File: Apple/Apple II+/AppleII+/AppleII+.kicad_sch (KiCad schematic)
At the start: 0 parts

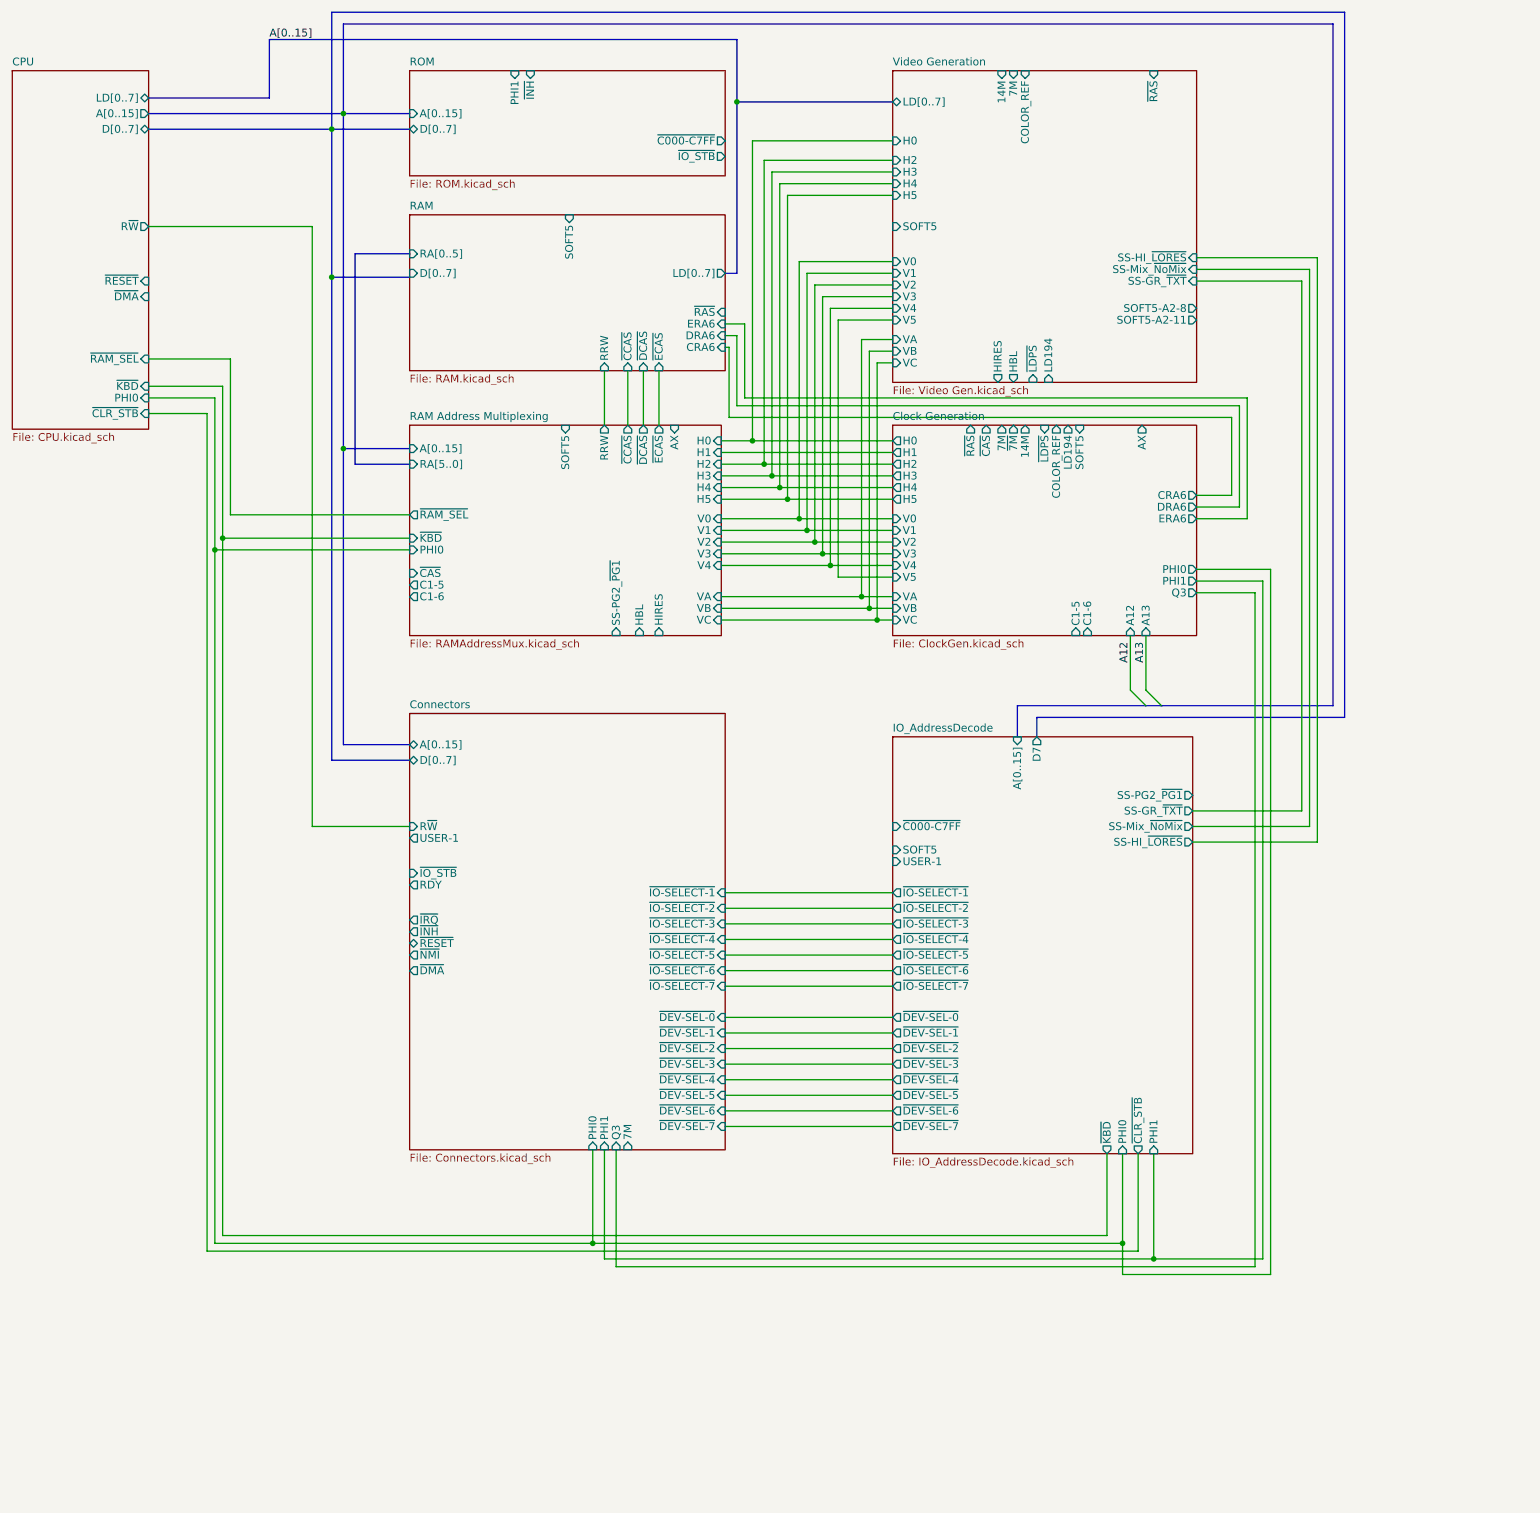
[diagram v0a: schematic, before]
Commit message: first time re-running ERC
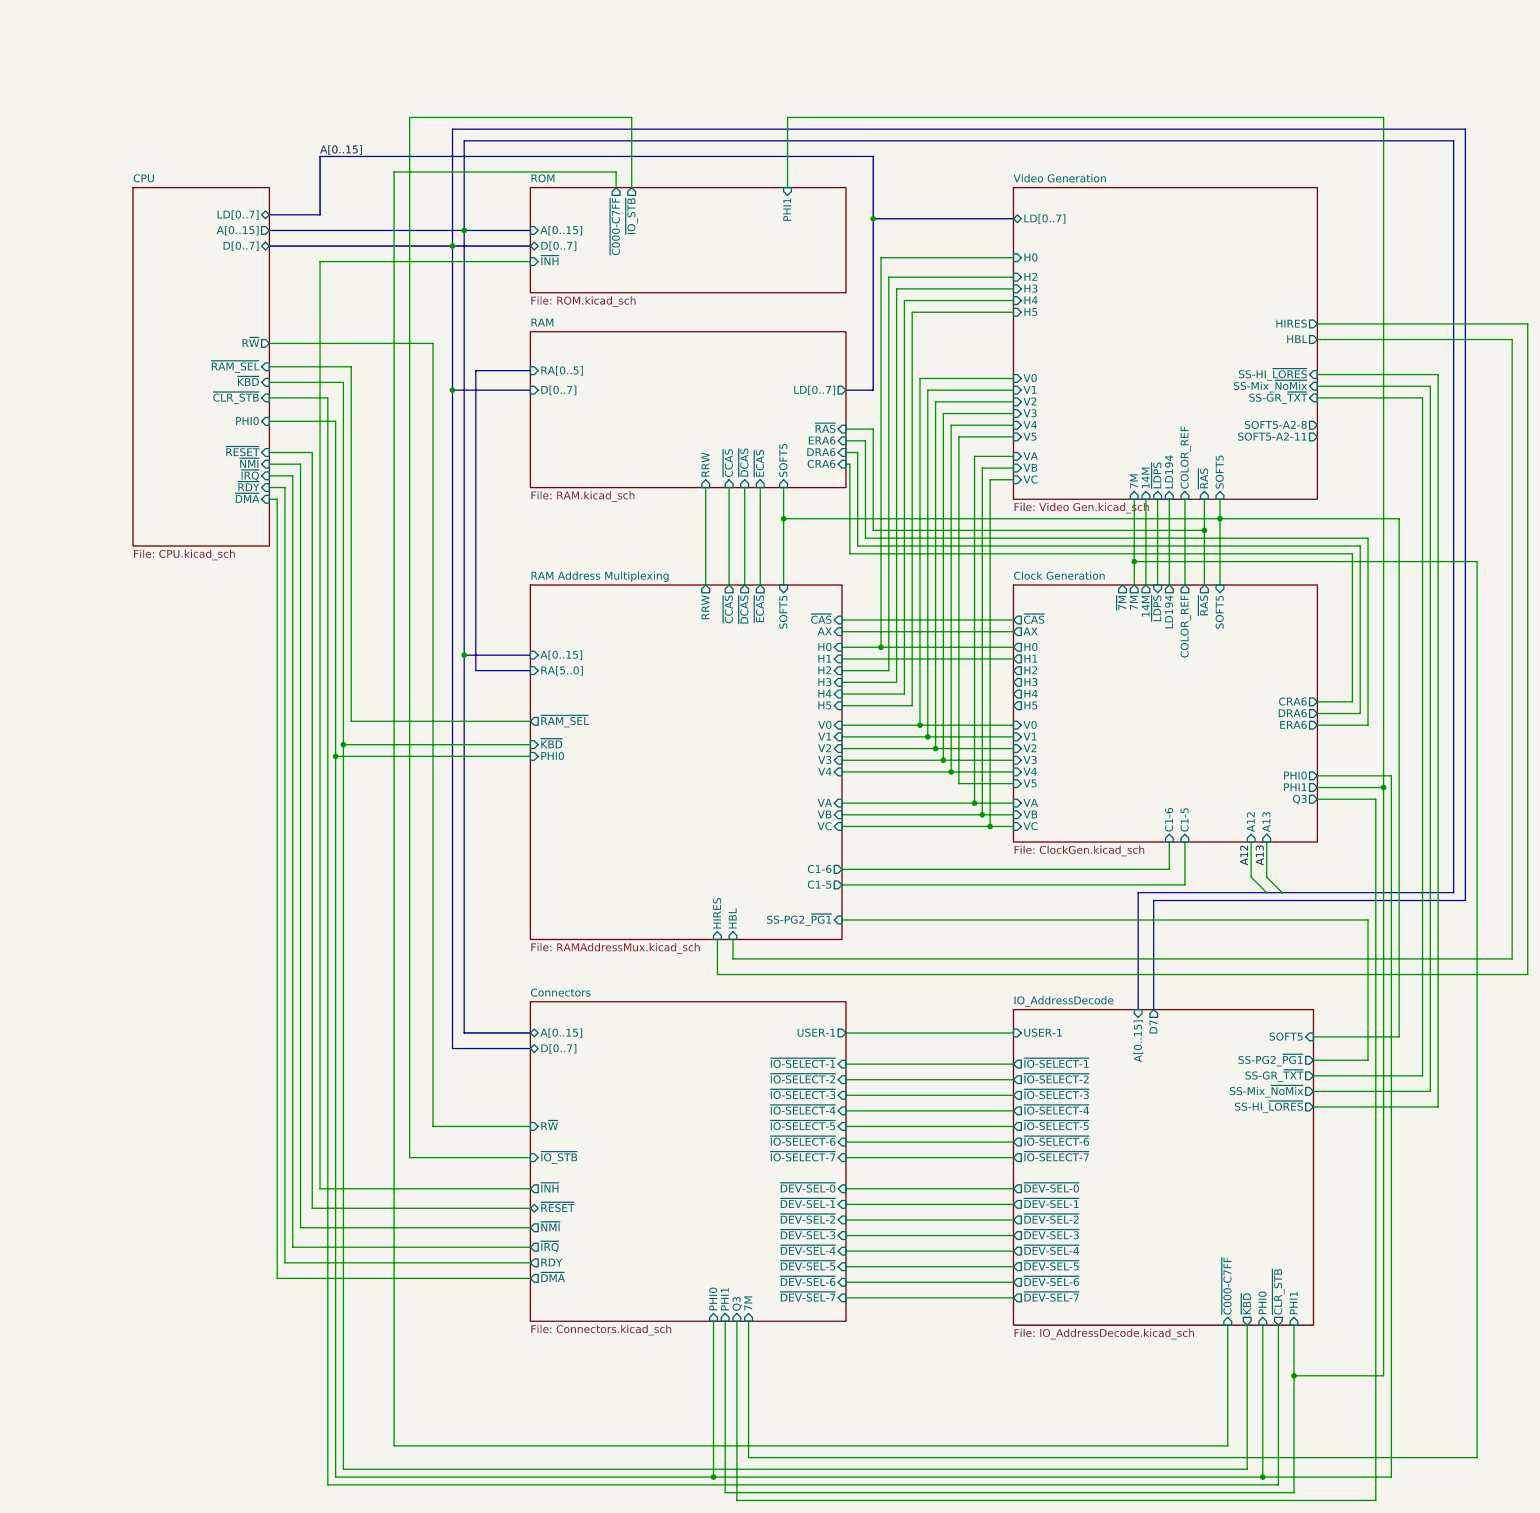
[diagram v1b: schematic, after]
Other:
- sheet CPU ports: added ~{IRQ}, ~{NMI}, ~{RDY}; removed none
